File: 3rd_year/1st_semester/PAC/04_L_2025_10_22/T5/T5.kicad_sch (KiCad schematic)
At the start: 13 parts

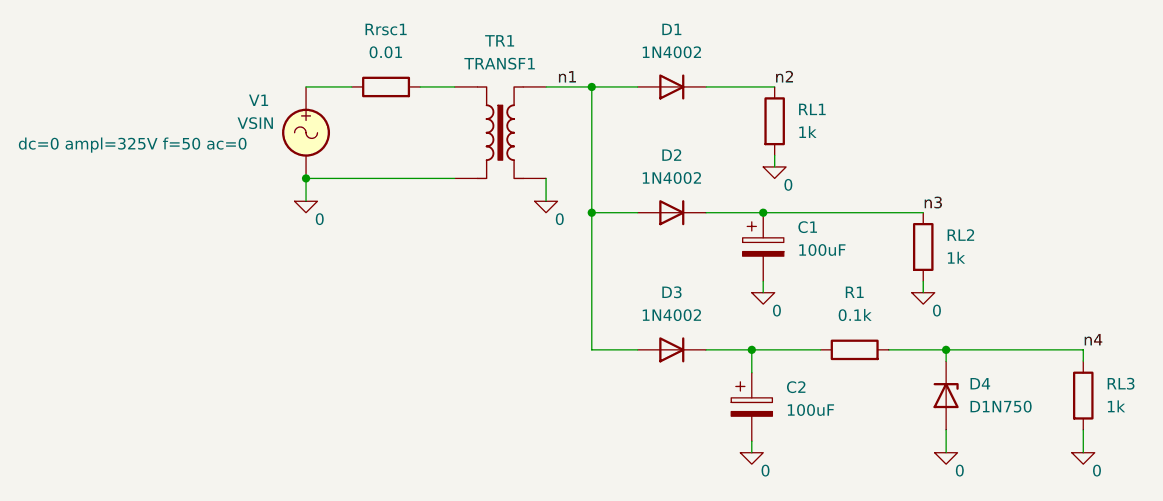
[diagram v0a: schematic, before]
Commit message: uncommited
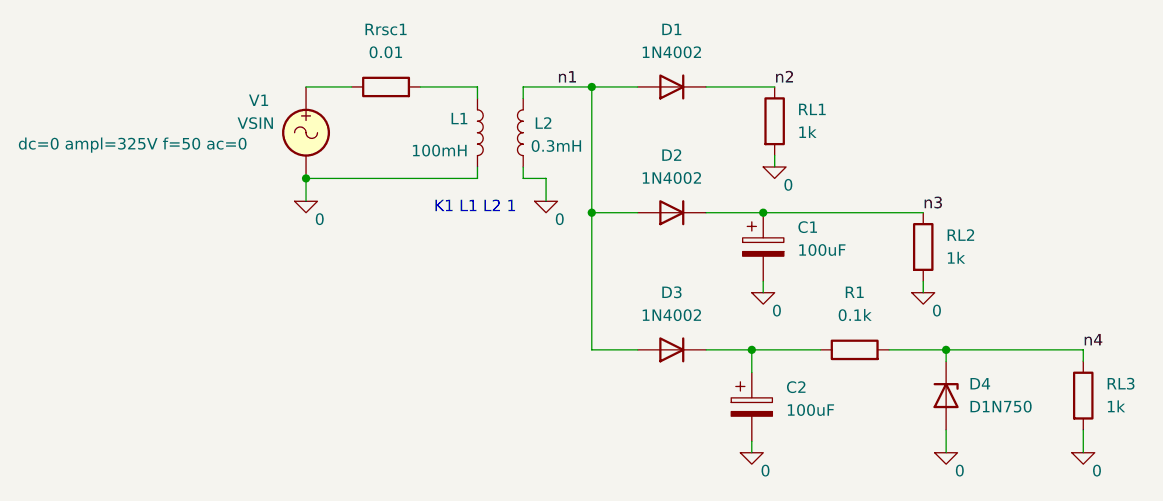
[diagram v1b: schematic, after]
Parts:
- removed TR1: TRANSF1, symbol Transformer:TRANSF1
- added L1: 100mH, symbol Device:L
- added L2: 0.3mH, symbol Device:L
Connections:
- net 0: now also L1.2, L2.2
- net n1: now also L2.1
- net at Rrsc1.2: now also L1.1
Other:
- note added: "K1 L1 L2 1"
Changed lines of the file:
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@@
 	(generator_version "9.0")
 	(paper "A4")
+	(text "K1 L1 L2 1"
+		(exclude_from_sim no)
+		(at 64.516 122.682 0)
+		(effects
+			(font
+				(size 1.27 1.27)
+			)
+		)
+	)
 	(junction
 		(at 77.47 109.22)
@@
 	(wire
 		(pts
+			(xy 69.85 118.11) (xy 69.85 119.38)
+		)
+		(stroke
+			(width 0)
+			(type default)
+		)
+	)
+	(wire
+		(pts
 			(xy 110.49 138.43) (xy 116.84 138.43)
 		)
@@
 	(wire
 		(pts
+			(xy 69.85 109.22) (xy 77.47 109.22)
+		)
+		(stroke
+			(width 0)
+			(type default)
+		)
+	)
+	(wire
+		(pts
 			(xy 90.17 123.19) (xy 96.52 123.19)
 		)
@@
 	(wire
 		(pts
-			(xy 45.72 119.38) (xy 62.23 119.38)
+			(xy 45.72 119.38) (xy 64.77 119.38)
 		)
 		(stroke
@@
 	(wire
 		(pts
+			(xy 69.85 119.38) (xy 72.39 119.38)
+		)
+		(stroke
+			(width 0)
+			(type default)
+		)
+	)
+	(wire
+		(pts
 			(xy 96.52 123.19) (xy 114.3 123.19)
 		)
@@
 	(wire
 		(pts
+			(xy 64.77 109.22) (xy 64.77 110.49)
+		)
+		(stroke
+			(width 0)
+			(type default)
+		)
+	)
+	(wire
+		(pts
 			(xy 77.47 109.22) (xy 82.55 109.22)
 		)
@@
 	(wire
 		(pts
+			(xy 69.85 109.22) (xy 69.85 110.49)
+		)
+		(stroke
+			(width 0)
+			(type default)
+		)
+	)
+	(wire
+		(pts
 			(xy 95.25 148.59) (xy 95.25 149.86)
 		)
@@
 	(wire
 		(pts
-			(xy 72.39 109.22) (xy 77.47 109.22)
+			(xy 64.77 118.11) (xy 64.77 119.38)
 		)
 		(stroke
@@
 	(wire
 		(pts
-			(xy 58.42 109.22) (xy 62.23 109.22)
+			(xy 58.42 109.22) (xy 64.77 109.22)
 		)
 		(stroke
@@
 	)
 	(symbol
+		(lib_id "Device:L")
+		(at 69.85 114.3 0)
+		(mirror y)
+		(unit 1)
+		(exclude_from_sim no)
+		(in_bom yes)
+		(on_board yes)
+		(dnp no)
+		(property "Reference" "L2"
+			(at 73.152 113.284 0)
+			(effects
+				(font
+					(size 1.27 1.27)
+				)
+				(justify left)
+			)
+		)
+		(property "Value" "0.3mH"
+			(at 76.454 115.824 0)
+			(effects
+				(font
+					(size 1.27 1.27)
+				)
+				(justify left)
+			)
+		)
+		(property "Footprint" ""
+			(at 69.85 114.3 0)
+			(effects
+				(font
+					(size 1.27 1.27)
+				)
+				(hide yes)
+			)
+		)
+		(property "Datasheet" "~"
+			(at 69.85 114.3 0)
+			(effects
+				(font
+					(size 1.27 1.27)
+				)
+				(hide yes)
+			)
+		)
+		(property "Description" "Inductor"
+			(at 69.85 114.3 0)
+			(effects
+				(font
+					(size 1.27 1.27)
+				)
+				(hide yes)
+			)
+		)
+		(pin "2"
+		)
+		(pin "1"
+		)
+		(instances
+			(project "T5"
+				(path "/49e4a9d4-e782-4d33-b9f7-63927972d99e"
+					(reference "L2")
+					(unit 1)
+				)
+			)
+		)
+	)
+	(symbol
 		(lib_id "Device:D_Zener")
 		(at 116.84 143.51 270)
@@
 	)
 	(symbol
-		(lib_id "Transformer:TRANSF1")
-		(at 67.31 114.3 0)
-		(unit 1)
-		(exclude_from_sim no)
-		(in_bom yes)
-		(on_board yes)
-		(dnp no)
-		(fields_autoplaced yes)
-		(property "Reference" "TR1"
-			(at 67.31 104.14 0)
-			(effects
-				(font
-					(size 1.27 1.27)
-				)
-			)
-		)
-		(property "Value" "TRANSF1"
-			(at 67.31 106.68 0)
-			(effects
-				(font
-					(size 1.27 1.27)
-				)
+		(lib_id "Device:L")
+		(at 64.77 114.3 0)
+		(unit 1)
+		(exclude_from_sim no)
+		(in_bom yes)
+		(on_board yes)
+		(dnp no)
+		(property "Reference" "L1"
+			(at 61.722 112.776 0)
+			(effects
+				(font
+					(size 1.27 1.27)
+				)
+				(justify left)
+			)
+		)
+		(property "Value" "100mH"
+			(at 57.404 116.332 0)
+			(effects
+				(font
+					(size 1.27 1.27)
+				)
+				(justify left)
 			)
 		)
 		(property "Footprint" ""
-			(at 67.31 114.3 0)
-			(effects
-				(font
-					(size 1.27 1.27)
-				)
-				(hide yes)
-			)
-		)
-		(property "Datasheet" ""
-			(at 67.31 114.3 0)
-			(effects
-				(font
-					(size 1.27 1.27)
-				)
-				(hide yes)
-			)
-		)
-		(property "Description" ""
-			(at 67.31 114.3 0)
-			(effects
-				(font
-					(size 1.27 1.27)
-				)
-				(hide yes)
-			)
-		)
-		(property "Sim.Device" "K"
-			(at 67.31 114.3 0)
-			(effects
-				(font
-					(size 1.27 1.27)
-				)
-				(hide yes)
-			)
-		)
-		(property "Sim.Params" "l1=100m l2=0.1m k=1"
-			(at 67.31 114.3 0)
-			(effects
-				(font
-					(size 1.27 1.27)
-				)
-				(hide yes)
-			)
-		)
-		(pin "3"
-		)
-		(pin "4"
-		)
-		(pin "1"
+			(at 64.77 114.3 0)
+			(effects
+				(font
+					(size 1.27 1.27)
+				)
+				(hide yes)
+			)
+		)
+		(property "Datasheet" "~"
+			(at 64.77 114.3 0)
+			(effects
+				(font
+					(size 1.27 1.27)
+				)
+				(hide yes)
+			)
+		)
+		(property "Description" "Inductor"
+			(at 64.77 114.3 0)
+			(effects
+				(font
+					(size 1.27 1.27)
+				)
+				(hide yes)
+			)
 		)
 		(pin "2"
 		)
+		(pin "1"
+		)
 		(instances
 			(project ""
 				(path "/49e4a9d4-e782-4d33-b9f7-63927972d99e"
-					(reference "TR1")
-					(unit 1)
-				)
+					(reference "L1")
+					(unit 1)
+				)
